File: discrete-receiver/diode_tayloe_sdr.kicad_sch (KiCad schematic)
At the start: 7 parts, among them J2 Optional 5V DC Jack, J3 USB_C_Receptacle_USB2.0_16P, J4 RJ45_Hanrun_HR911105A_Horizon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, U9 LAN8720A

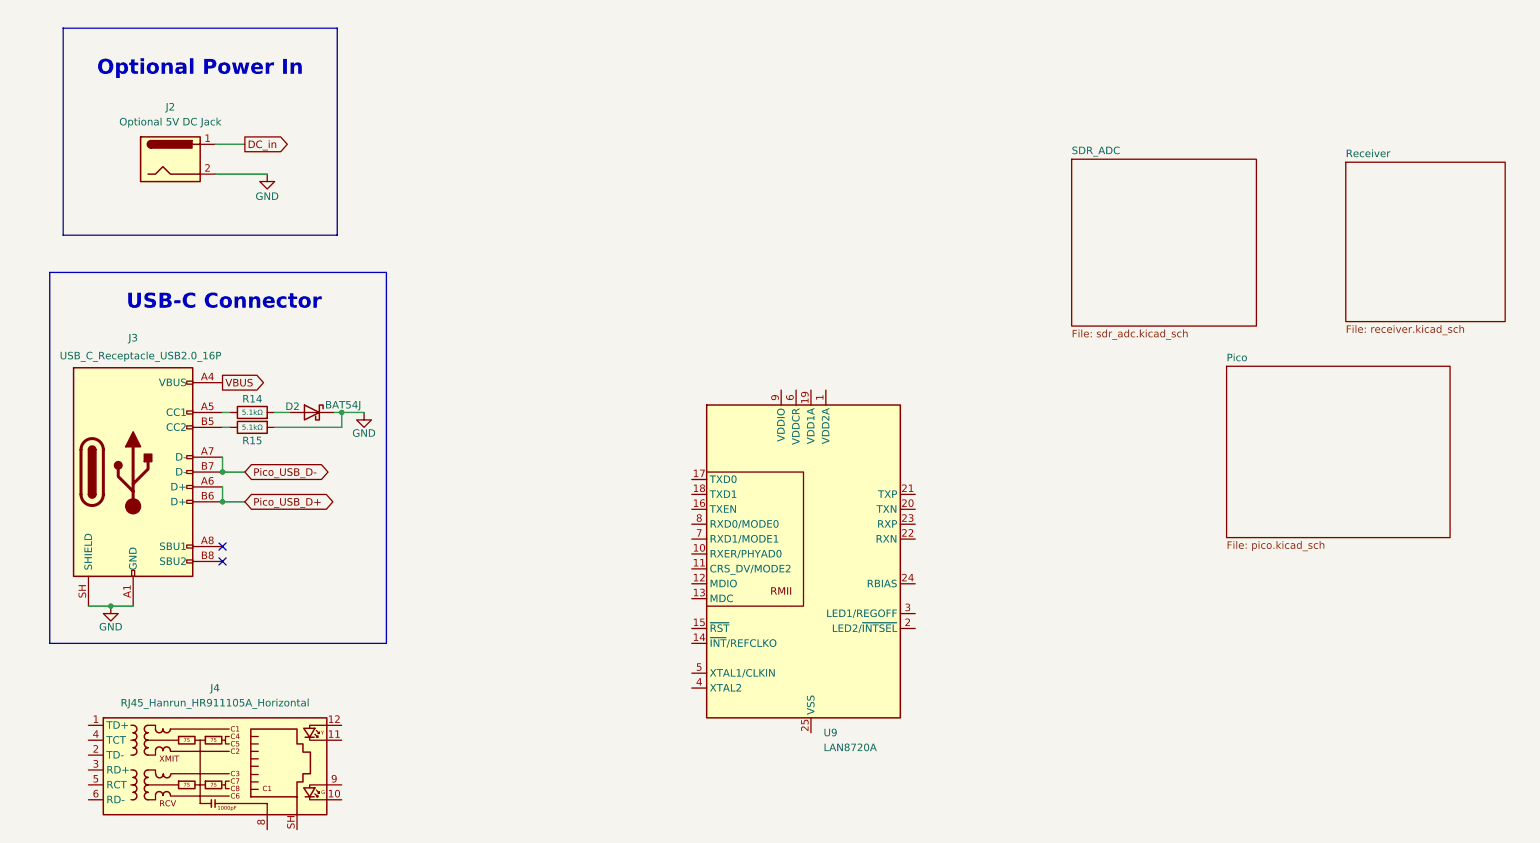
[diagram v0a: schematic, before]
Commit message: update schematic for peter
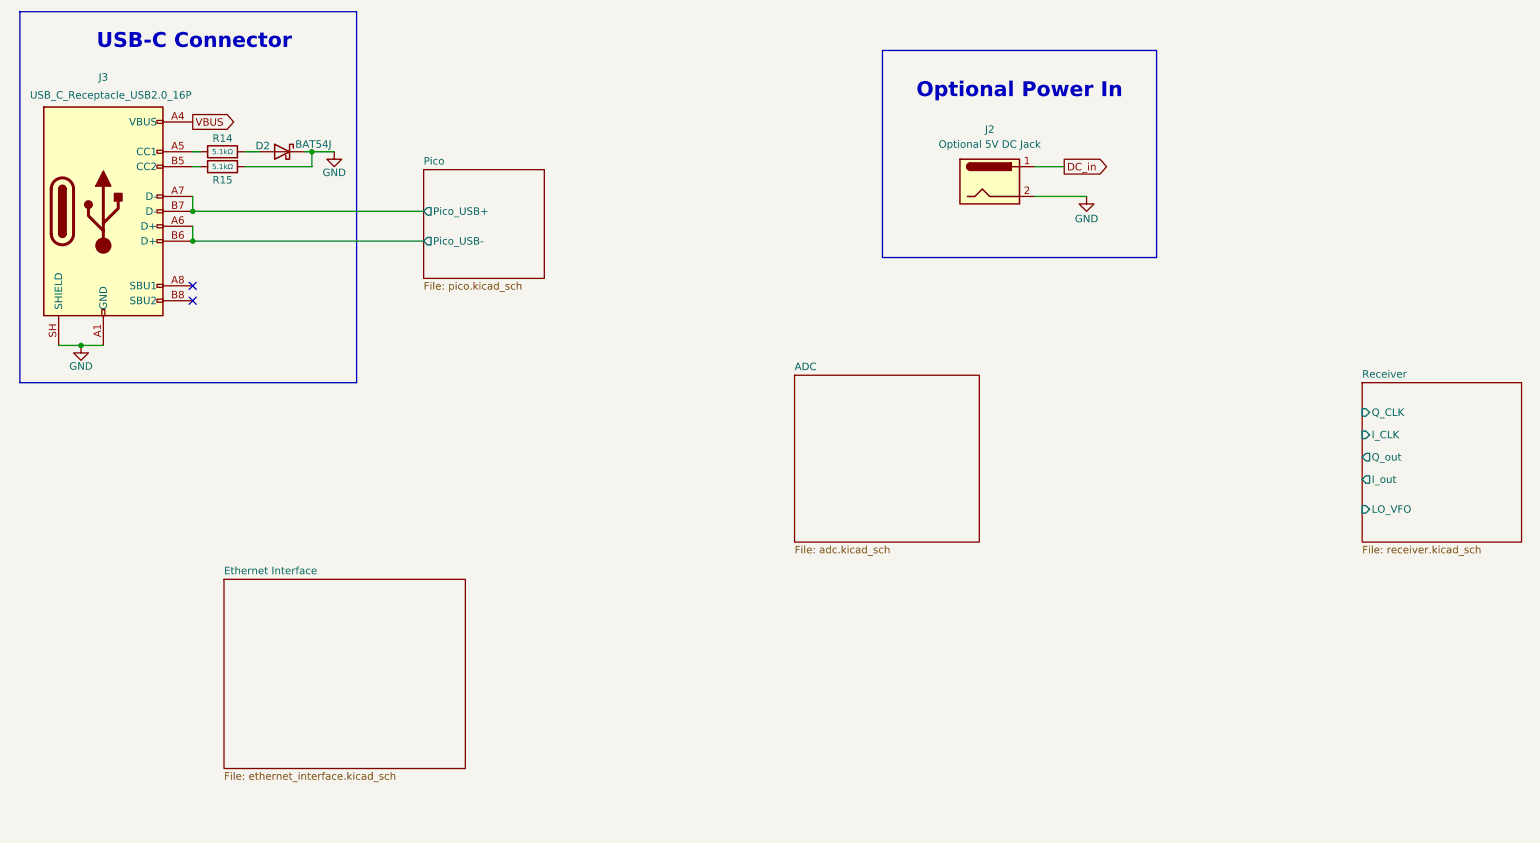
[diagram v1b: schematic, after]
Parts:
- removed J4: RJ45_Hanrun_HR911105A_Horizontal, Connector_RJ:RJ45_Hanrun_HR911105A_Horizontal, symbol Connector:RJ45_Hanrun_HR911105A_Horizontal
- removed U9: LAN8720A, Package_DFN_QFN:VQFN-24-1EP_4x4mm_P0.5mm_EP2.5x2.5mm_ThermalVias, symbol Interface_Ethernet:LAN8720A
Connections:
- net Pico_USB_D+ renamed Pico/Pico_USB-
- net Pico_USB_D- renamed Pico/Pico_USB+
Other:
- sheet SDR_ADC renamed ADC
- added sheet Ethernet Interface (ethernet_interface.kicad_sch)
- sheet ADC: file sdr_adc.kicad_sch -> adc.kicad_sch
- sheet Pico ports: added Pico_USB+, Pico_USB-; removed none
- sheet Receiver ports: added I_CLK, I_out, LO_VFO, Q_CLK, Q_out; removed none
- moved on the sheet: D2, J2, J3, R14, R15
